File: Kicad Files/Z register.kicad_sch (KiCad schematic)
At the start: 25 parts, among them SW3 SW_DIP_x02, U15 74LS00, U16 LM555xN, U17 74LS273, U18 74LS112, U19 74LS112, U20 28C256, U21 74LS139, U22 HDSP-7403, U23 HDSP-7403, U24 HDSP-7403, U25 HDSP-7403

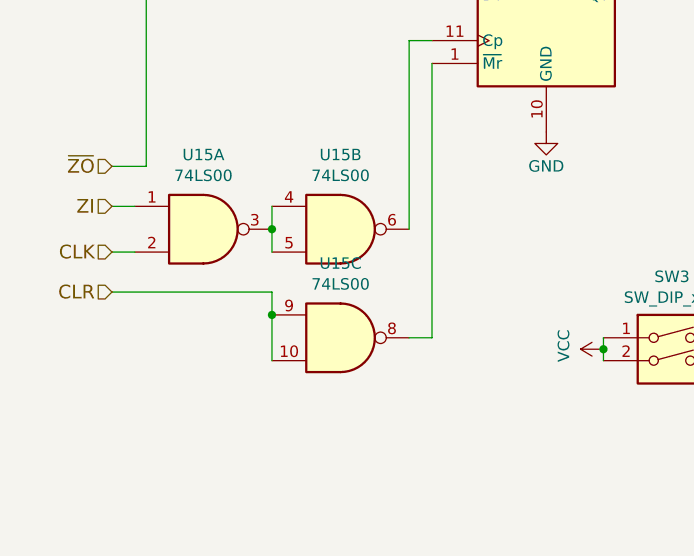
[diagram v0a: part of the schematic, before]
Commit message: update
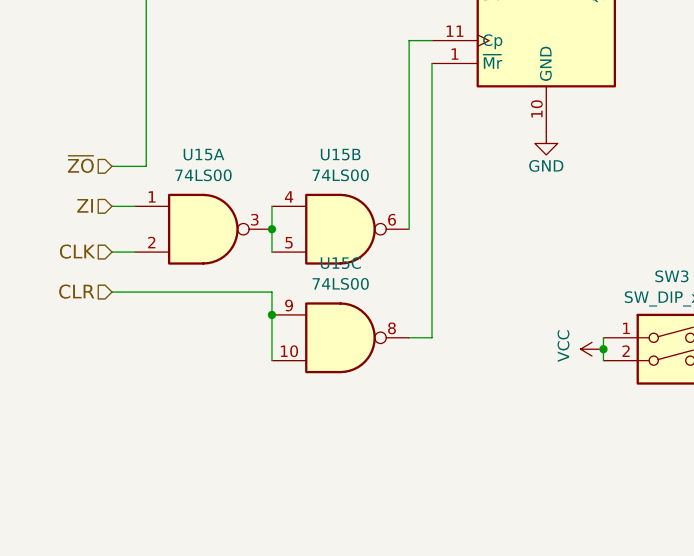
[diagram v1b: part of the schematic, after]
